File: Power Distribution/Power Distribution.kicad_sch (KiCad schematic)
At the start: 14 parts, among them P1 Charging/BoostConverterBoardT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, U2 Raspberryt Pi Zero 2W

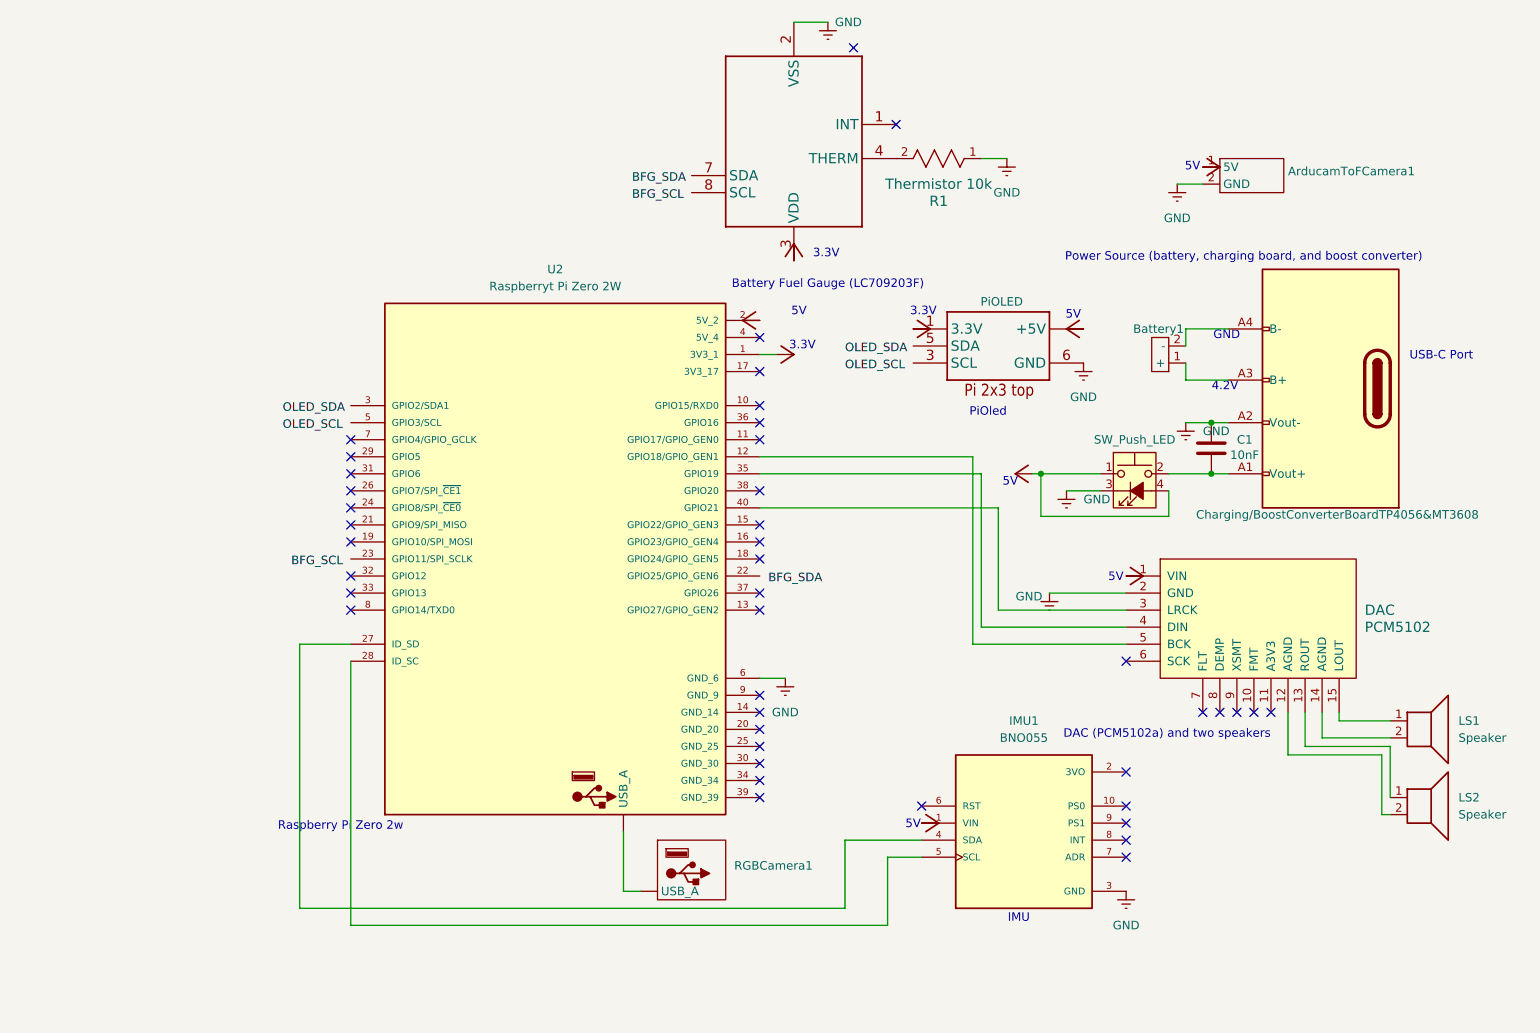
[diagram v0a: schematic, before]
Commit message: PCB
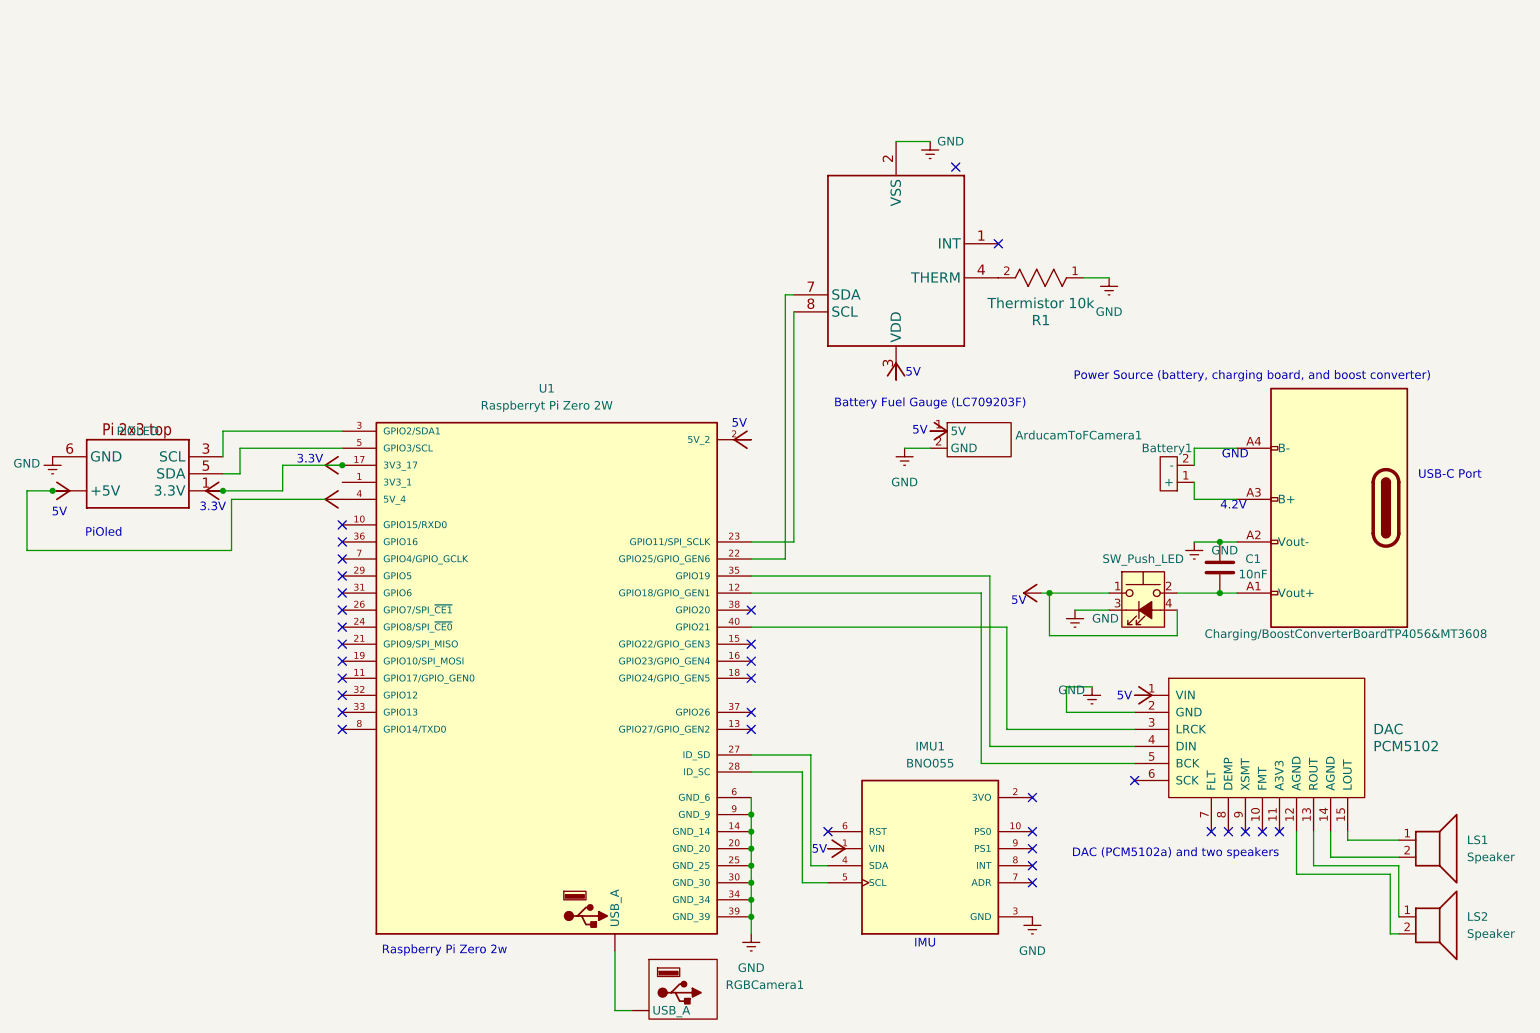
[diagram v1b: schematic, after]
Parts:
- removed U2: Raspberryt Pi Zero 2W, Raspberry Pi Zero 2 w:MODULE_SC1176, symbol SC1176:SC1176
- added U1: Raspberryt Pi Zero 2W, Raspberry Pi Zero 2 w:MODULE_SC1176, symbol SC1176:SC1176
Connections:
- net GND: now also U1.14 (GND_14), U1.20 (GND_20), U1.25 (GND_25), U1.30 (GND_30), U1.34 (GND_34), U1.39 (GND_39), U1.6 (GND_6), U1.9 (GND_9)
- net at 1.7 (SDA): now also U1.22 (GPIO25/GPIO_GEN6)
- net at 1.8 (SCL): now also U1.23 (GPIO11/SPI_SCLK)
- net at RGBCamera1. (USB_A): now also U1. (USB_A)
- net at DAC.5 (BCK): now also U1.12 (GPIO18/GPIO_GEN1)
- net at IMU1.4 (SDA): now also U1.27 (ID_SD)
- net at IMU1.5 (SCL): now also U1.28 (ID_SC)
- net at DAC.4 (DIN): now also U1.35 (GPIO19)
- net at DAC.3 (LRCK): now also U1.40 (GPIO21)
- net at PiOLED.1 (3.3V): now also U1.17 (3V3_17)
- net at PiOLED.3 (SCL): now also U1.3 (GPIO2/SDA1)
- net at PiOLED.5 (SDA): now also U1.5 (GPIO3/SCL)
- no-connect marks 42 -> 33
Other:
- moved on the sheet: ArducamToFCamera1, Battery1, C1, DAC, IMU1, LS1, LS2, PiOLED, R1, RGBCamera1
